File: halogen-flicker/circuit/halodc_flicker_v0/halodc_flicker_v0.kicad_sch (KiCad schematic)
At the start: 21 parts, among them J1 SPI, J2 Conn_01x02_Pin, J3 Conn_01x02_Pin, Q1 IRF540N, SW1 SW_DIP_x02, SW2 SW_Push, U1 ATtiny13A-S, U2 PC817, U3 AMS1117-5.0

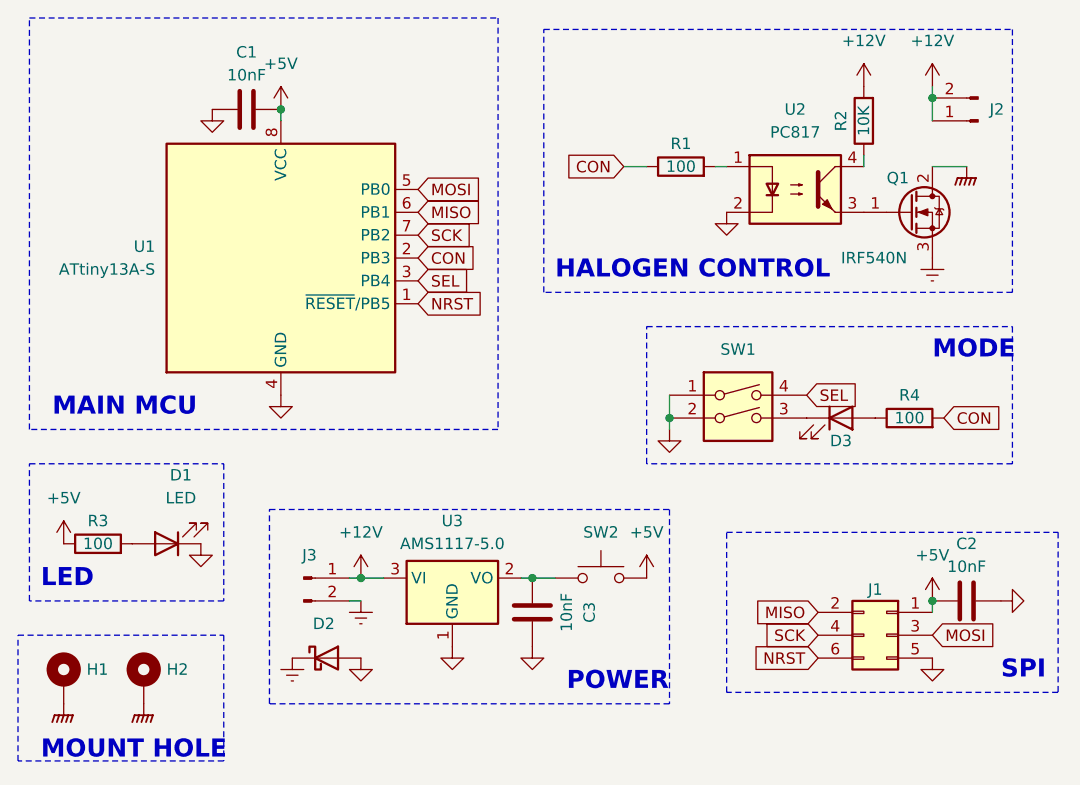
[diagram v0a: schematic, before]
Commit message: Halogen FLicker
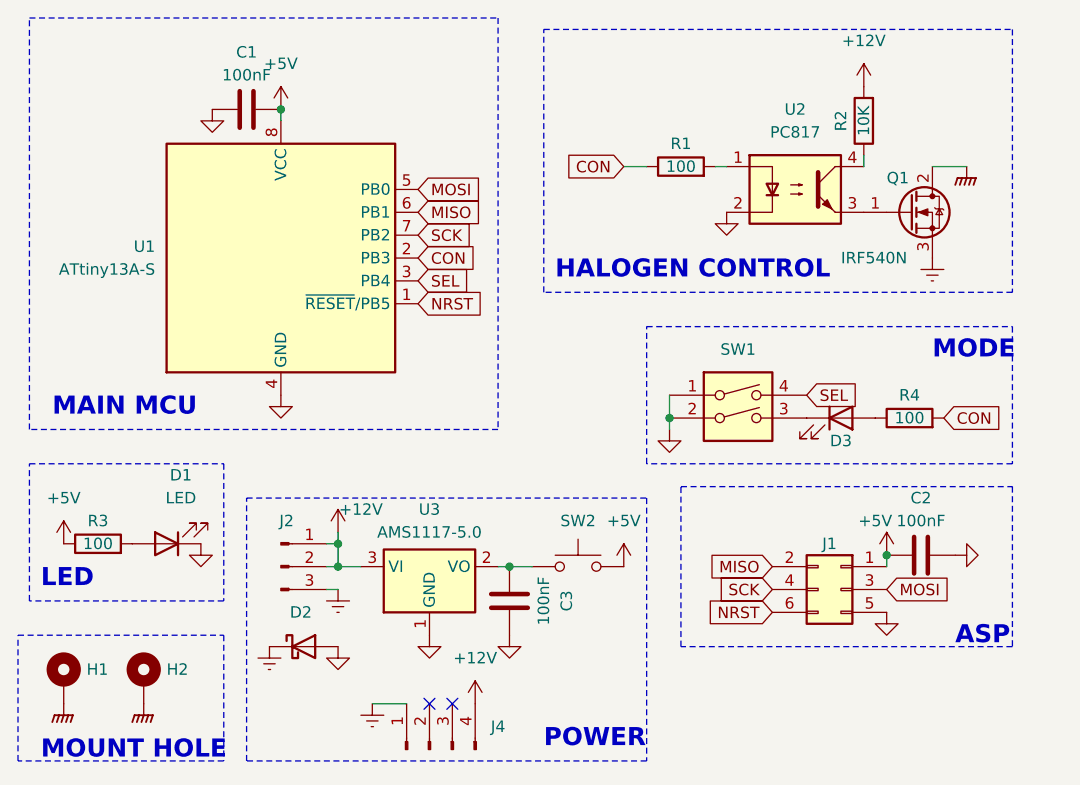
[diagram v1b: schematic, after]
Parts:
- removed J2, J3: Conn_01x02_Pin, symbol Connector:Conn_01x02_Pin
- added J2: BATT_LAMP, TerminalBlock:TerminalBlock_Altech_AK300-3_P5.00mm, symbol Connector:Conn_01x03_Pin
- added J4: CHARGER, Connector_Molex:Molex_KK-254_AE-6410-04A_1x04_P2.54mm_Vertical, symbol Connector:Conn_01x04_Pin
- C1, C2, C3: value 10nF -> 100nF; footprint (none) -> Capacitor_SMD:C_0805_2012Metric_Pad1.18x1.45mm_HandSolder
- D1, D3: footprint (none) -> LED_SMD:LED_0805_2012Metric_Pad1.15x1.40mm_HandSolder
- D2: footprint (none) -> Diode_SMD:D_SMB-SMC_Universal_Handsoldering
- H1, H2: footprint (none) -> MountingHole:MountingHole_4.5mm_Pad
- J1: value SPI -> ASP; footprint (none) -> Connector_PinHeader_2.54mm:PinHeader_2x03_P2.54mm_Vertical
- Q1: footprint Package_TO_SOT_THT:TO-220-3_Vertical -> Package_TO_SOT_THT:TO-220-3_Horizontal_TabDown
- R1, R2, R3, R4: footprint (none) -> Resistor_SMD:R_0805_2012Metric_Pad1.20x1.40mm_HandSolder
- SW1: footprint (none) -> Button_Switch_THT:SW_DIP_SPSTx02_Slide_9.78x7.26mm_W7.62mm_P2.54mm
- SW2: footprint (none) -> Button_Switch_THT:SW_Tactile_SPST_Angled_PTS645Vx31-2LFS
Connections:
- net +12V: now also J2.1 (Pin_1), J2.2 (Pin_2), J4.4 (Pin_4)
- net GNDREF: now also J2.3 (Pin_3), J4.1 (Pin_1)
- no-connect marks 0 -> 2
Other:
- note added: "ASP"
- note removed: "SPI"
- moved on the sheet: C2, C3, D2, J1, SW2, U3
